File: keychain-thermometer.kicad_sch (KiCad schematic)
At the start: 4 parts, among them U1 ATtiny85V-10S

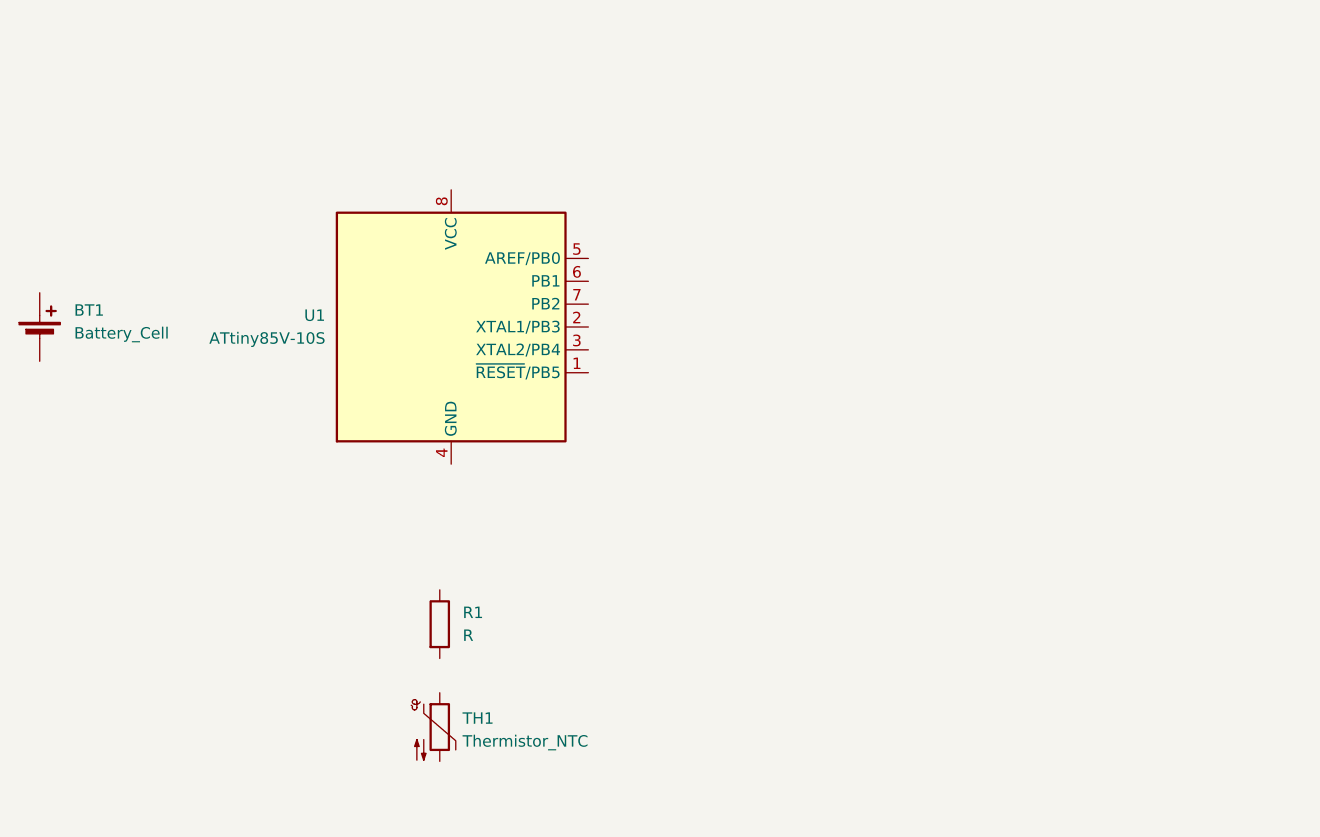
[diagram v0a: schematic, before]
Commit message: first commit, started drawing schematic
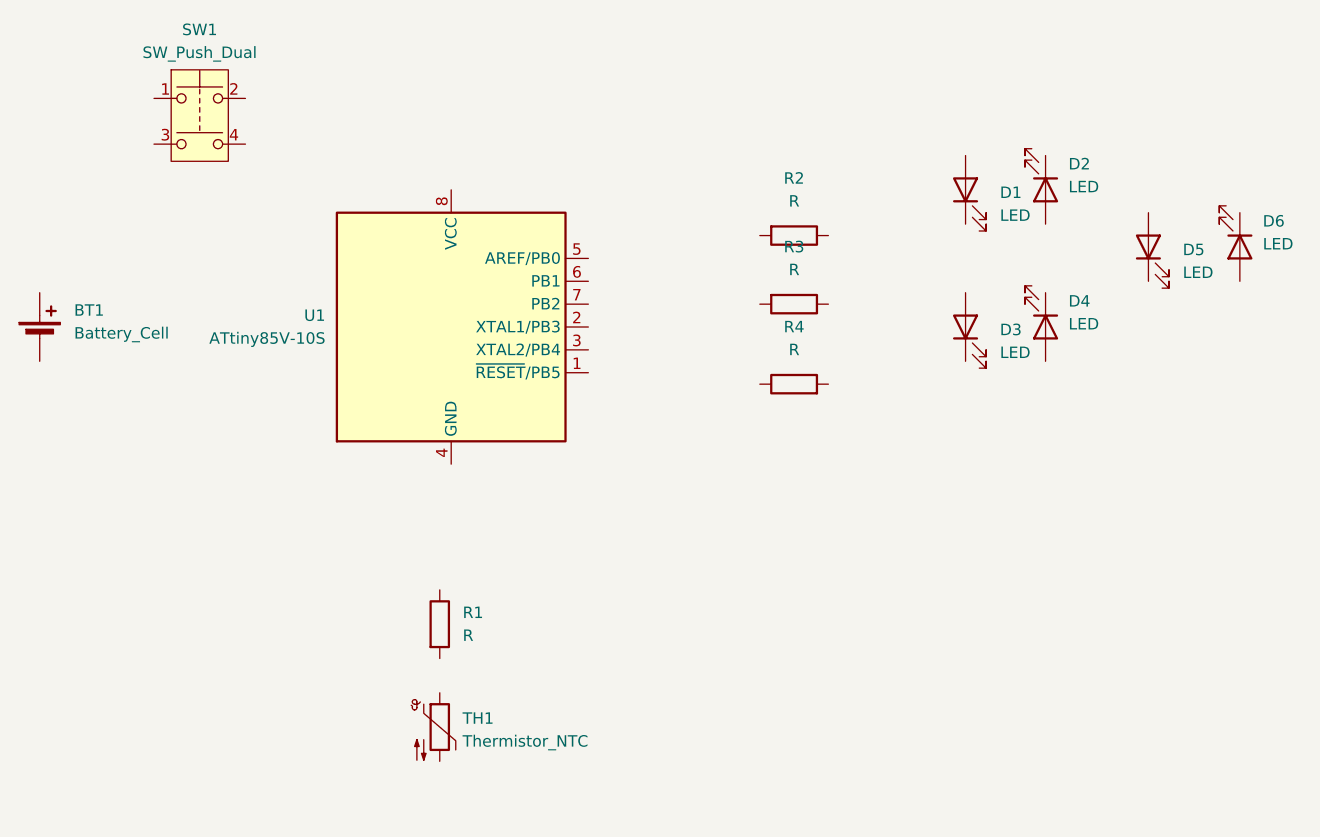
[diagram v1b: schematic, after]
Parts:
- added D1, D2, D3, D4, D5, D6: LED, symbol Device:LED
- added R2, R3, R4: R, symbol Device:R
- added SW1: SW_Push_Dual, symbol Switch:SW_Push_Dual

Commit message: creared PCB and started routing
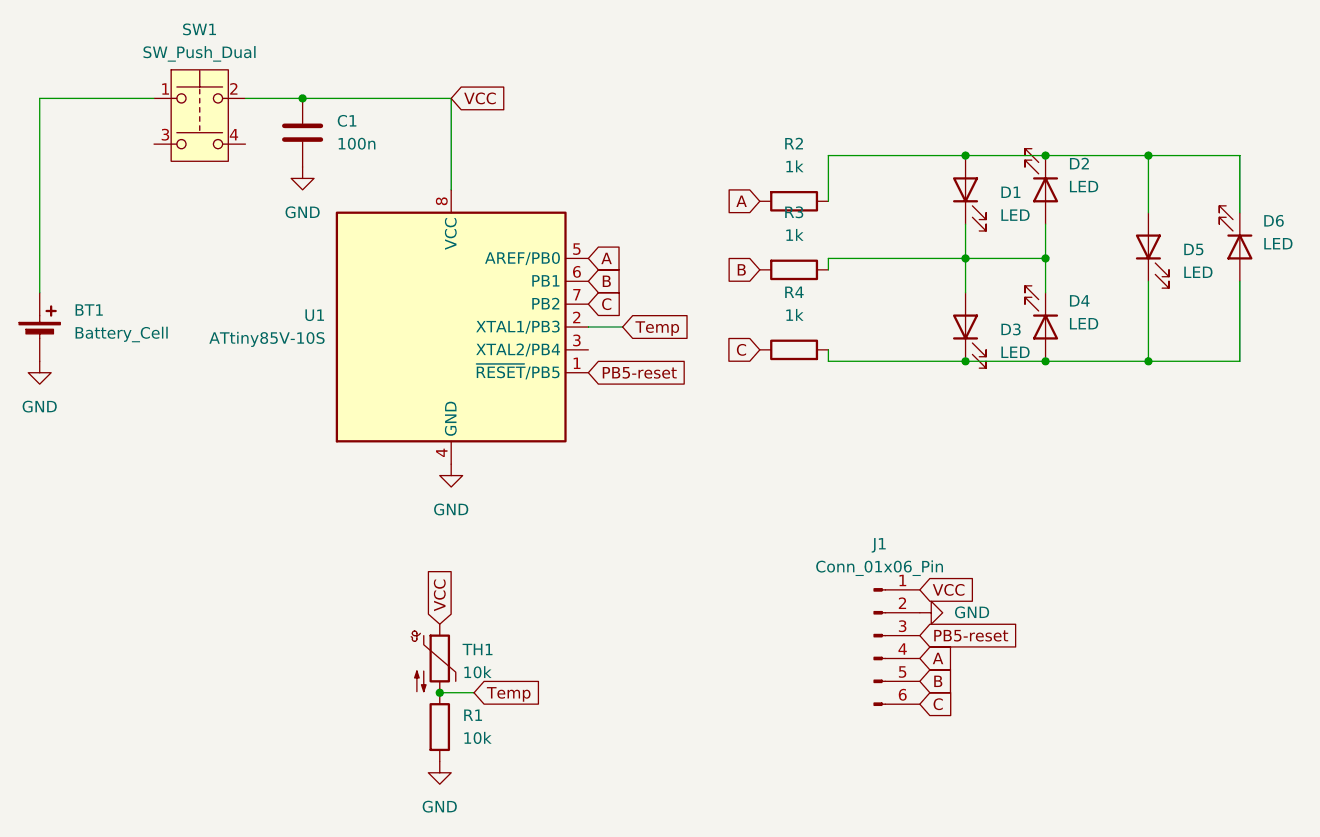
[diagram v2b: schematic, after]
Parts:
- added C1: 100n, Capacitor_SMD:C_0805_2012Metric, symbol Device:C
- added J1: Conn_01x06_Pin, Connector_PinHeader_2.54mm:PinHeader_1x06_P2.54mm_Vertical, symbol Connector:Conn_01x06_Pin
- BT1: footprint (none) -> Battery:Battery_Panasonic_CR2032-HFN_Horizontal_CircularHoles
- D1, D2, D3, D4, D5, D6: footprint (none) -> LED_SMD:LED_0805_2012Metric
- R1: value R -> 10k; footprint (none) -> Resistor_SMD:R_0805_2012Metric
- R2, R3, R4: value R -> 1k; footprint (none) -> Resistor_SMD:R_0805_2012Metric
- SW1: footprint (none) -> Button_Switch_SMD:SW_SPST_PTS810
- TH1: value Thermistor_NTC -> 10k; footprint (none) -> Resistor_SMD:R_0805_2012Metric
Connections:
- net at D6.1 (K): now also D1.2 (A), D2.1 (K), D5.2 (A), R2.1
- net at D6.2 (A): now also D3.1 (K), D4.2 (A), D5.1 (K), R4.2
- net at BT1.1 (+): now also SW1.1
- net GND: now reaches BT1.2 (-)
- net GND: now also R1.2, U1.4 (GND), C1.2, J1.2 (Pin_2)
- net PB5-reset: now reaches U1.1 (~{RESET}/PB5)
- net PB5-reset: now also J1.3 (Pin_3)
- net Temp: now reaches U1.2 (XTAL1/PB3)
- net Temp: now also R1.1, TH1.2
- net A: now reaches U1.5 (AREF/PB0)
- net A: now also R2.2, J1.4 (Pin_4)
- net B: now reaches U1.6 (PB1)
- net B: now also R3.2, J1.5 (Pin_5)
- net C: now reaches U1.7 (PB2)
- net C: now also R4.1, J1.6 (Pin_6)
- net VCC: now reaches U1.8 (VCC)
- net VCC: now also SW1.2, TH1.1, C1.1, J1.1 (Pin_1)
- net at D1.1 (K): now also D2.2 (A), D3.2 (A), D4.1 (K), R3.1
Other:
- moved on the sheet: R1, R2, R3, R4, TH1
